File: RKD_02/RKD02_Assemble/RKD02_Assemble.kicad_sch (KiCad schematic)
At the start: 164 parts, among them J1 Qwiic_RA, J2 Qwiic_RA, M1 Mark, M2 Mark, M3 Mark, M4 Mark, M5 Mark, M6 Mark, M7 Mark, SW1 SW_Push, SW10 SW_Push, SW11 SW_Push, SW12 SW_Push, SW13 SW_Push, SW14 SW_Push, SW15 SW_Push, SW16 SW_Push, SW17 SW_Push, SW18 SW_Push, SW19 SW_Push, SW2 SW_Push, SW20 SW_Push, SW21 SW_Push, SW22 SW_Push, SW23 SW_Push, SW24 SW_Push, SW25 SW_Push, SW26 SW_Push, SW27 SW_Push, SW28 SW_Push, SW29 SW_Push, SW3 SW_Push, SW30 SW_Push, SW31 SW_Push, SW32 SW_Push, SW33 SW_Push, SW34 SW_Push, SW35 SW_Push, SW36 RotaryEncoder_Switch, SW4 SW_Push, SW40 RotaryEncoder_Switch, SW5 SW_Push, SW51 SW_Push, SW52 SW_Push, SW53 SW_Push, SW54 SW_Push, SW55 SW_Push, SW56 SW_Push, SW57 SW_Push, SW58 SW_Push, SW59 SW_Push, SW6 SW_Push, SW60 SW_Push, SW61 SW_Push, SW62 SW_Push, SW63 SW_Push, SW64 SW_Push, SW65 SW_Push, SW66 SW_Push, SW67 SW_Push, SW68 SW_Push, SW69 SW_Push, SW7 SW_Push, SW70 SW_Push, SW71 SW_Push, SW72 SW_Push, SW73 SW_Push, SW74 SW_Push, SW75 SW_Push, SW76 SW_Push, SW77 SW_Push, SW78 SW_Push, SW79 SW_Push, SW8 SW_Push, SW80 SW_Push, SW81 SW_Push, SW82 SW_Push, SW83 SW_Push, SW84 SW_Push, SW85 SW_Push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

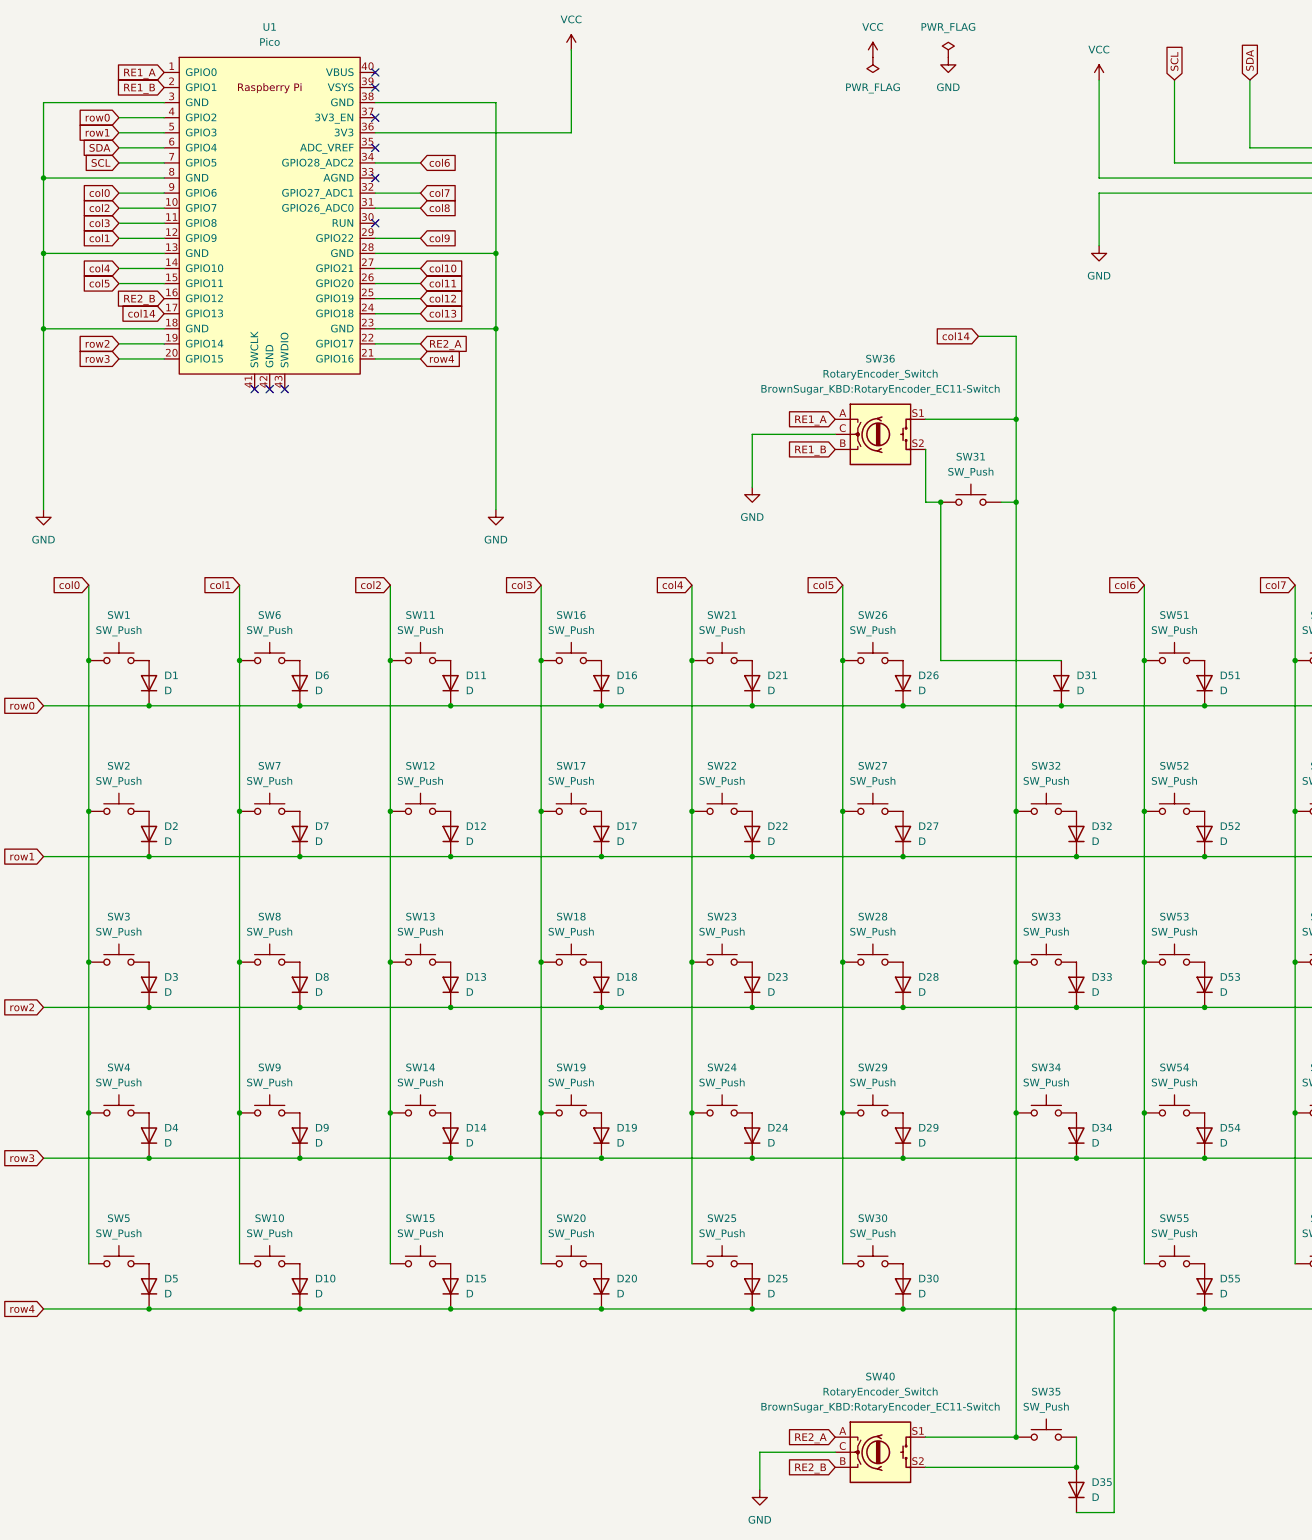
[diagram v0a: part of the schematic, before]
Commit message: RKD02 大量に調整
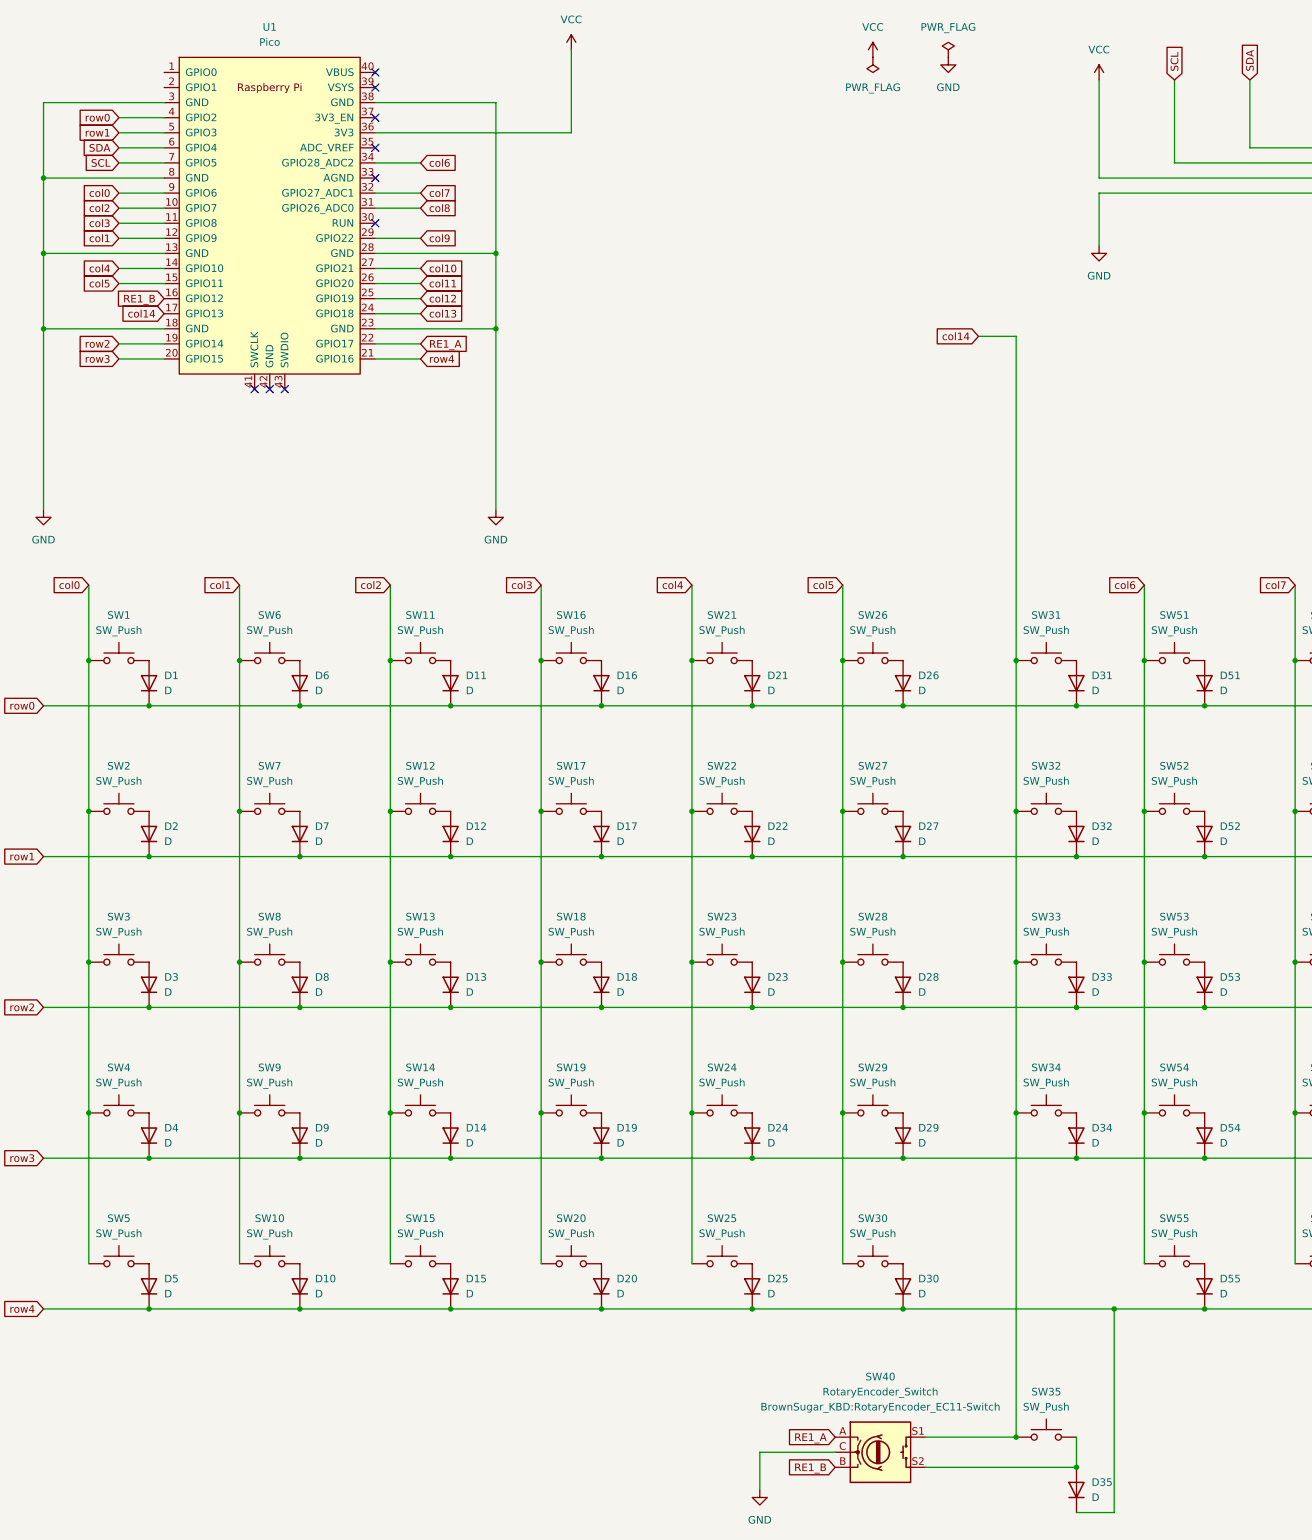
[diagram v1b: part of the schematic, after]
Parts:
- removed SW36: RotaryEncoder_Switch, BrownSugar_KBD:RotaryEncoder_EC11-Switch, symbol Device:RotaryEncoder_Switch
- SW31: footprint BrownSugar_KBD:SW_PUSH_6x3mm -> Rikkodo_FootPrint:rkd_Asm_ChocV1V2_Hotswap_1u
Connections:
- net RE2_A is gone; now on net RE1_A: SW40.A, U1.22 (GPIO17)
- net RE2_B is gone; now on net RE1_B: SW40.B, U1.16 (GPIO12)
- net RE1_A: no longer U1.1 (GPIO0)
- net RE1_B: no longer U1.2 (GPIO1)
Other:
- moved on the sheet: D31, SW31
